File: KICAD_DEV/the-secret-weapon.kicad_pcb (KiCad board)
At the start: 6 copper layers, 150 x 150 mm, 2 parts, among them U1 STM32H743VITx, U2 USBLC6-2SC6

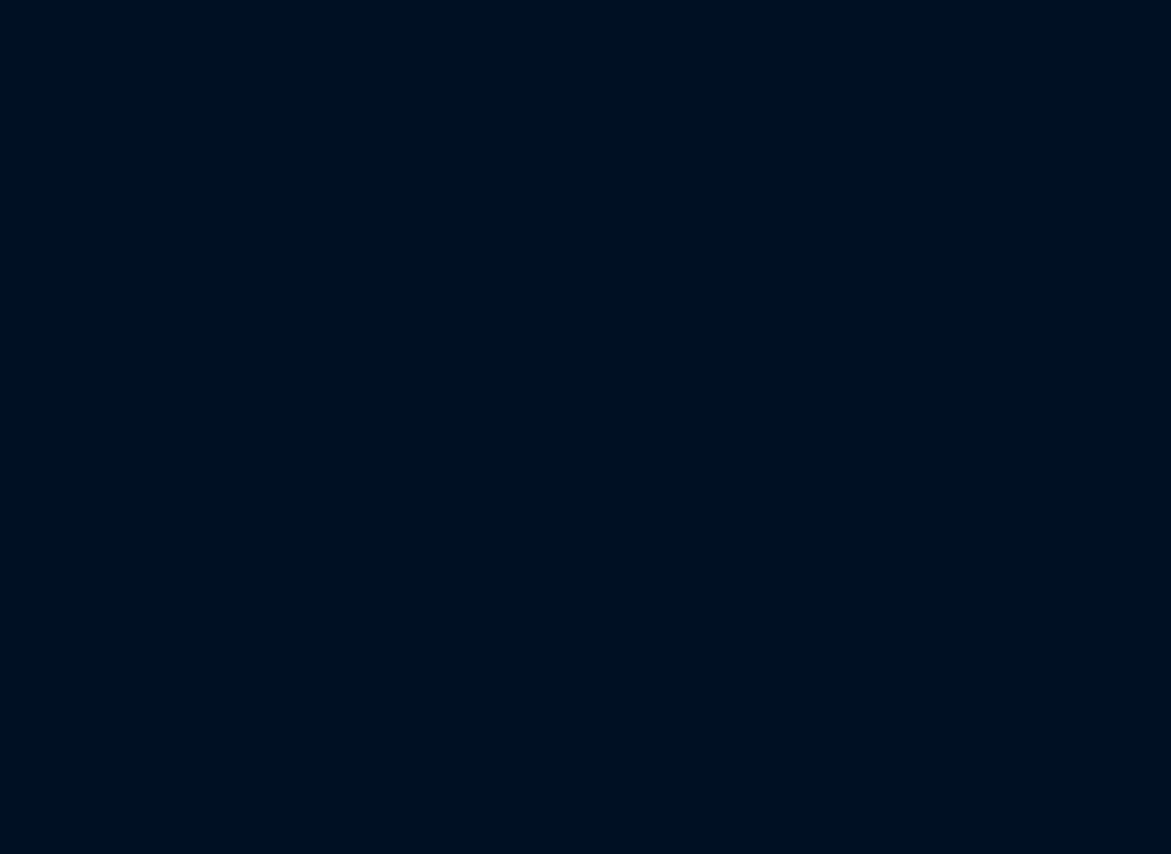
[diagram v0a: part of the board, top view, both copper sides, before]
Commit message: starting the actual board!
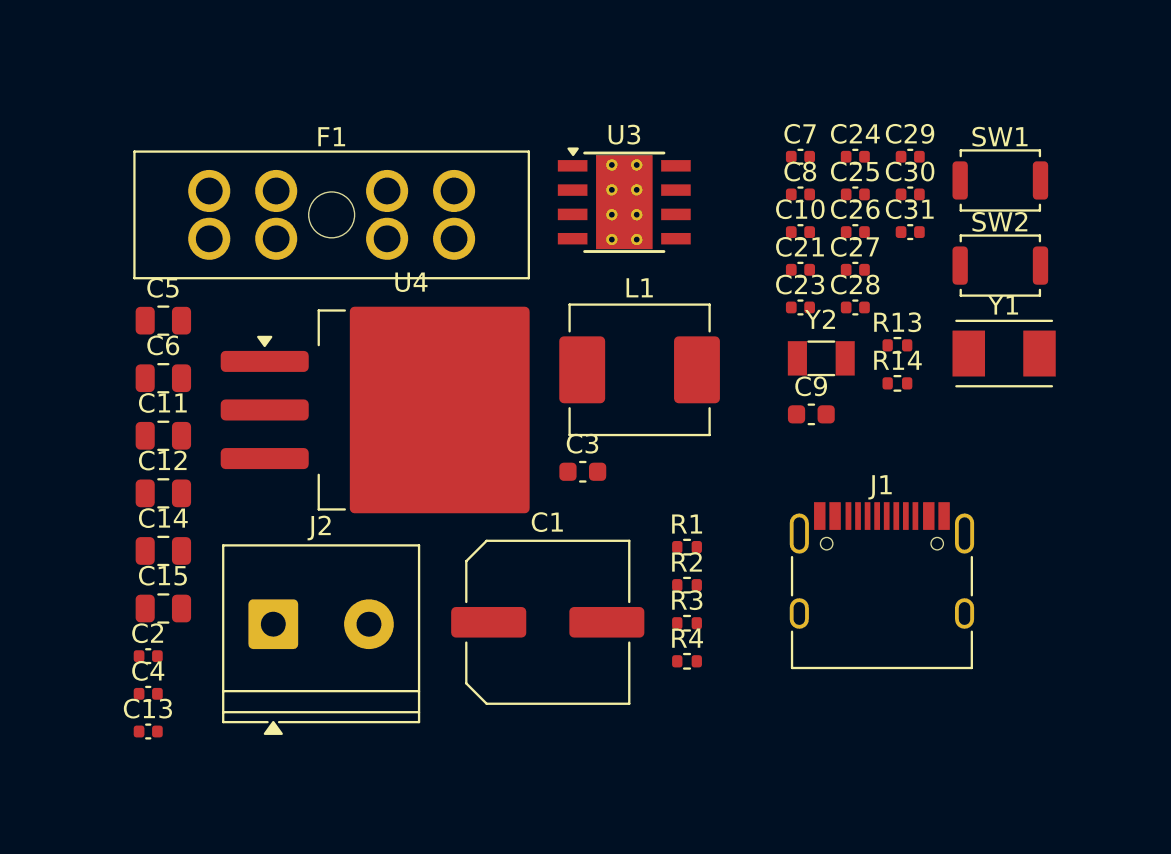
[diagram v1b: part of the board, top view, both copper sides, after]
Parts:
- added C1: 100uF, Capacitor_SMD:C_Elec_8x6.2, F.Cu at (103.2, 91.0)
- added C10: 0.1uF, Capacitor_SMD:C_0402_1005Metric, F.Cu at (116.4, 70.6)
- added C11: 22uF, Capacitor_SMD:C_0805_2012Metric, F.Cu at (83.1, 81.2)
- added C12: 22uF, Capacitor_SMD:C_0805_2012Metric, F.Cu at (83.1, 84.2)
- added C13: 1uF, Capacitor_SMD:C_0402_1005Metric, F.Cu at (82.3, 96.7)
- added C14: 10uF, Capacitor_SMD:C_0805_2012Metric, F.Cu at (83.1, 87.2)
- added C15: 22uF, Capacitor_SMD:C_0805_2012Metric, F.Cu at (83.1, 90.2)
- added C2: 220nF, Capacitor_SMD:C_0402_1005Metric, F.Cu at (82.3, 92.7)
- added C21: 0.1uF, Capacitor_SMD:C_0402_1005Metric, F.Cu at (116.4, 72.5)
- added C23: 0.1uF, Capacitor_SMD:C_0402_1005Metric, F.Cu at (116.4, 74.5)
- added C24: 0.1uF, Capacitor_SMD:C_0402_1005Metric, F.Cu at (119.3, 66.6)
- added C25: 0.1uF, Capacitor_SMD:C_0402_1005Metric, F.Cu at (119.3, 68.6)
- added C26: 0.1uF, Capacitor_SMD:C_0402_1005Metric, F.Cu at (119.3, 70.6)
- added C27: 0.1uF, Capacitor_SMD:C_0402_1005Metric, F.Cu at (119.3, 72.5)
- added C28: 32pF, Capacitor_SMD:C_0402_1005Metric, F.Cu at (119.3, 74.5)
- added C29: 32pF, Capacitor_SMD:C_0402_1005Metric, F.Cu at (122.2, 66.6)
- added C3: 10uF, Capacitor_SMD:C_0603_1608Metric, F.Cu at (105.0, 83.1)
- added C30: 17pF, Capacitor_SMD:C_0402_1005Metric, F.Cu at (122.2, 68.6)
- added C31: 17pF, Capacitor_SMD:C_0402_1005Metric, F.Cu at (122.2, 70.6)
- added C4: 0.1uF, Capacitor_SMD:C_0402_1005Metric, F.Cu at (82.3, 94.7)
- added C5: 22uF, Capacitor_SMD:C_0805_2012Metric, F.Cu at (83.1, 75.2)
- added C6: 22uF, Capacitor_SMD:C_0805_2012Metric, F.Cu at (83.1, 78.2)
- added C7: 2.2uF, Capacitor_SMD:C_0402_1005Metric, F.Cu at (116.4, 66.6)
- added C8: 2.2uF, Capacitor_SMD:C_0402_1005Metric, F.Cu at (116.4, 68.6)
- added C9: 4.7uF, Capacitor_SMD:C_0603_1608Metric, F.Cu at (117.0, 80.1)
- added F1: 20A, Fuse:FuseHolder_Blade_ATO_Littelfuse_FLR_178.6165, F.Cu at (85.5, 68.4)
- added J1: USB_C_Receptacle_USB2.0_14P, Connector_USB:USB_C_Receptacle_HRO_TYPE-C-31-M-12, F.Cu at (120.7, 89.5)
- added J2: Screw_Terminal_01x02, TerminalBlock_Phoenix:TerminalBlock_Phoenix_PT-1,5-2-5.0-H_1x02_P5.00mm_Horizontal, F.Cu at (88.9, 91.1)
- added L1: 6.8uH, Inductor_SMD:L_TechFuse_SL0650, F.Cu at (108.0, 77.8)
- added R1: 5.1K, Resistor_SMD:R_0402_1005Metric, F.Cu at (110.5, 87.0)
- added R13: 10K, Resistor_SMD:R_0402_1005Metric, F.Cu at (121.5, 76.5)
- added R14: 10K, Resistor_SMD:R_0402_1005Metric, F.Cu at (121.5, 78.5)
- added R2: 5.1K, Resistor_SMD:R_0402_1005Metric, F.Cu at (110.5, 89.0)
- added R3: 100K, Resistor_SMD:R_0402_1005Metric, F.Cu at (110.5, 91.0)
- added R4: 24.9K, Resistor_SMD:R_0402_1005Metric, F.Cu at (110.5, 93.0)
- added SW1: SW_Push, Button_Switch_SMD:SW_Push_SPST_NO_Alps_SKRK, F.Cu at (126.9, 67.9)
- added SW2: SW_Push, Button_Switch_SMD:SW_Push_SPST_NO_Alps_SKRK, F.Cu at (126.9, 72.3)
- added U3: LMR33640ADDA, Package_SO:Texas_HSOP-8-1EP_3.9x4.9mm_P1.27mm_ThermalVias, F.Cu at (107.2, 69.0)
- added U4: LM1086S-3.3/TR, Package_TO_SOT_SMD:TO-263-3_TabPin2, F.Cu at (96.1, 79.9)
- added Y1: 8 MHz, Crystal:Crystal_SMD_TXC_7A-2Pin_5x3.2mm, F.Cu at (127.1, 76.9)
- added Y2: 32.768 KHz, Crystal:Crystal_SMD_3215-2Pin_3.2x1.5mm, F.Cu at (117.5, 77.2)
